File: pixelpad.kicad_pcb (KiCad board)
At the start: 2 copper layers, 19 x 57 mm, 4 parts, among them SW1 SW_Push, SW2 SW_Push, SW3 SW_Push, U1 MOUDLE-SEEEDUINO-XIAO

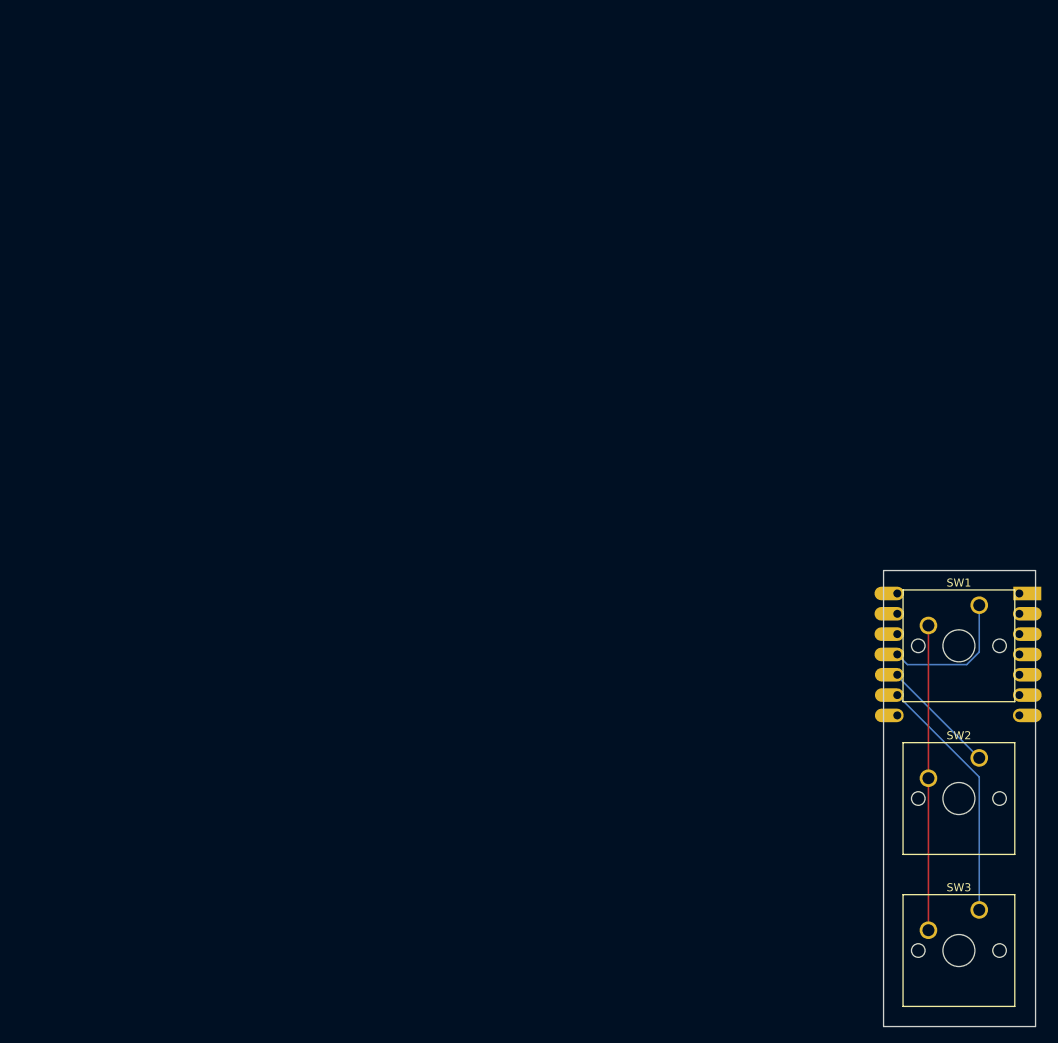
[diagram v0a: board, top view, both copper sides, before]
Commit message: Added stuff to the pcb editor
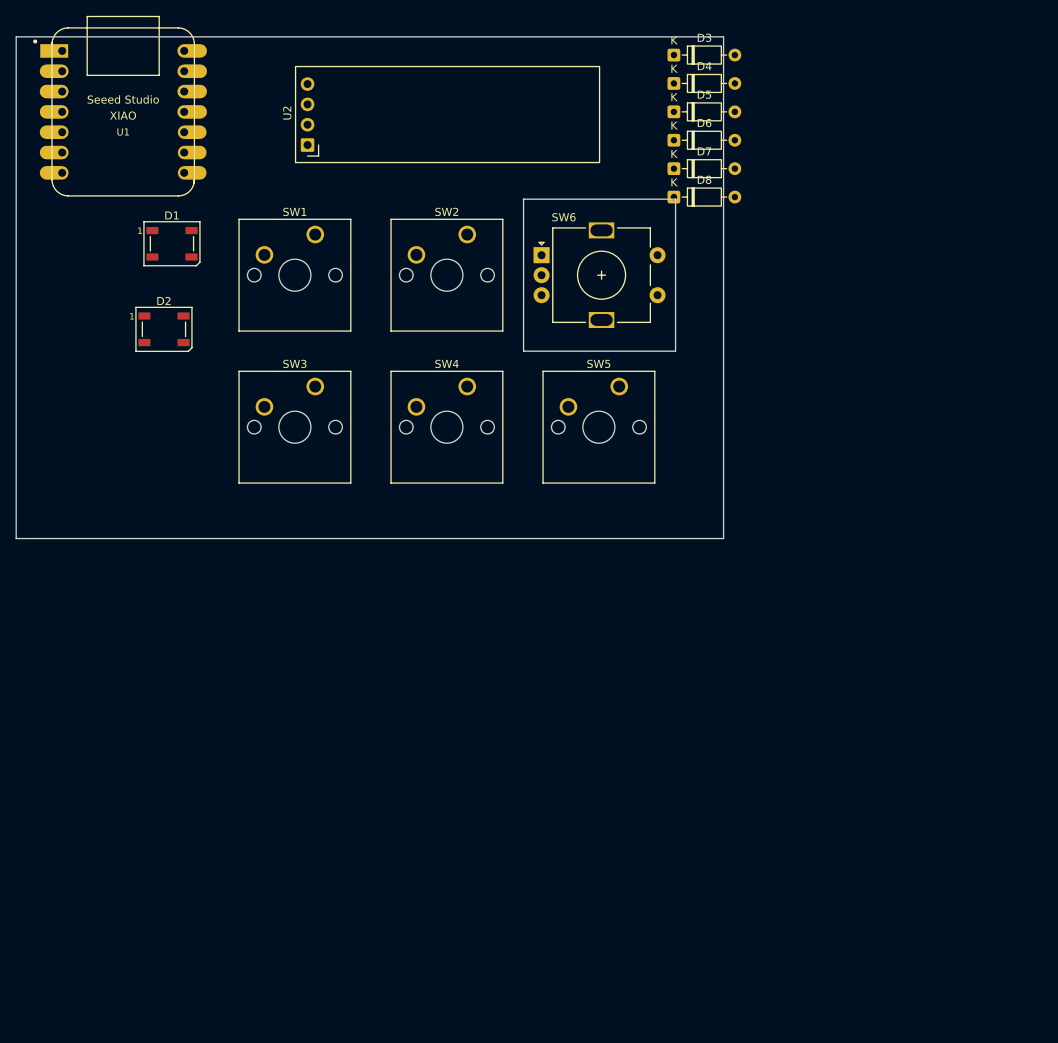
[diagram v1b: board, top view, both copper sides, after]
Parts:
- added D1: WS2812B, LED_SMD:LED_WS2812B_PLCC4_5.0x5.0mm_P3.2mm, F.Cu at (56.5, 45.1)
- added D2: WS2812B, LED_SMD:LED_WS2812B_PLCC4_5.0x5.0mm_P3.2mm, F.Cu at (55.5, 55.9)
- added D3: 1N914, Diode_THT:D_DO-35_SOD27_P7.62mm_Horizontal, F.Cu at (119.3, 21.6)
- added D4: 1N914, Diode_THT:D_DO-35_SOD27_P7.62mm_Horizontal, F.Cu at (119.3, 25.1)
- added D5: 1N914, Diode_THT:D_DO-35_SOD27_P7.62mm_Horizontal, F.Cu at (119.3, 28.7)
- added D6: 1N914, Diode_THT:D_DO-35_SOD27_P7.62mm_Horizontal, F.Cu at (119.3, 32.2)
- added D7: 1N914, Diode_THT:D_DO-35_SOD27_P7.62mm_Horizontal, F.Cu at (119.3, 35.8)
- added D8: 1N914, Diode_THT:D_DO-35_SOD27_P7.62mm_Horizontal, F.Cu at (119.3, 39.3)
- added SW4: SW_Push_45deg, Button_Switch_Keyboard:SW_Cherry_MX_1.00u_PCB, F.Cu at (93.5, 63.0)
- added SW5: SW_Push_45deg, Button_Switch_Keyboard:SW_Cherry_MX_1.00u_PCB, F.Cu at (112.5, 63.0)
- added SW6: RotaryEncoder_Switch, Rotary_Encoder:RotaryEncoder_Alps_EC11E-Switch_Vertical_H20mm, F.Cu at (102.8, 46.6)
- added U2: ER_OLEDM0.91_1x-I2C, Display:ER_OLEDM0.91_1x-I2C, F.Cu at (73.5, 32.8)
- SW1, SW2, SW3: value SW_Push -> SW_Push_45deg
- U1: moved to F.Cu
- moved U1 124.5 mm to (50.5, 28.7), turned to 0 degrees
- moved SW3 105.7 mm to (74.5, 63.0)
- moved SW1 95.1 mm to (74.5, 44.0)
- moved SW2 91.5 mm to (93.5, 44.0)
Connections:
- SW1 pad 1: Net-(U1-PA6_A10_D10_MOSI) -> COL0
- SW1 pad 2: GND -> Net-(D4-A)
- SW2 pad 1: Net-(U1-PA5_A9_D9_MISO) -> COL1
- SW2 pad 2: GND -> Net-(D5-A)
- SW3 pad 1: Net-(U1-PA7_A8_D8_SCK) -> COL2
- SW3 pad 2: GND -> Net-(D8-A)
- U1 pad 1: unconnected-(U1-PA02_A0_D0-Pad1) -> COL1
- U1 pad 10: Net-(U1-PA5_A9_D9_MISO) -> COL2
- U1 pad 11: Net-(U1-PA6_A10_D10_MOSI) -> unconnected-(U1-PA6_A10_D10_MOSI-Pad11)
- U1 pad 14: unconnected-(U1-5V-Pad14) -> VCC
- U1 pad 2: unconnected-(U1-PA4_A1_D1-Pad2) -> COL0
- U1 pad 3: unconnected-(U1-PA10_A2_D2-Pad3) -> ROW1
- U1 pad 4: unconnected-(U1-PA11_A3_D3-Pad4) -> ROW0
- U1 pad 5: unconnected-(U1-PA8_A4_D4_SDA-Pad5) -> SDA
- U1 pad 6: unconnected-(U1-PA9_A5_D5_SCL-Pad6) -> SCL
- U1 pad 8: unconnected-(U1-PB09_A7_D7_RX-Pad8) -> EC11B
- U1 pad 9: Net-(U1-PA7_A8_D8_SCK) -> EC11A
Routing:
- net GND: track 38.1 -> 0.00 mm
- net Net-(U1-PA7_A8_D8_SCK): track 31.1 -> 0.00 mm
- net Net-(U1-PA6_A10_D10_MOSI): track 17.6 -> 0.00 mm
- net Net-(U1-PA5_A9_D9_MISO): track 14.6 -> 0.00 mm
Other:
- board size 19 x 57 mm -> 88.4 x 62.7 mm

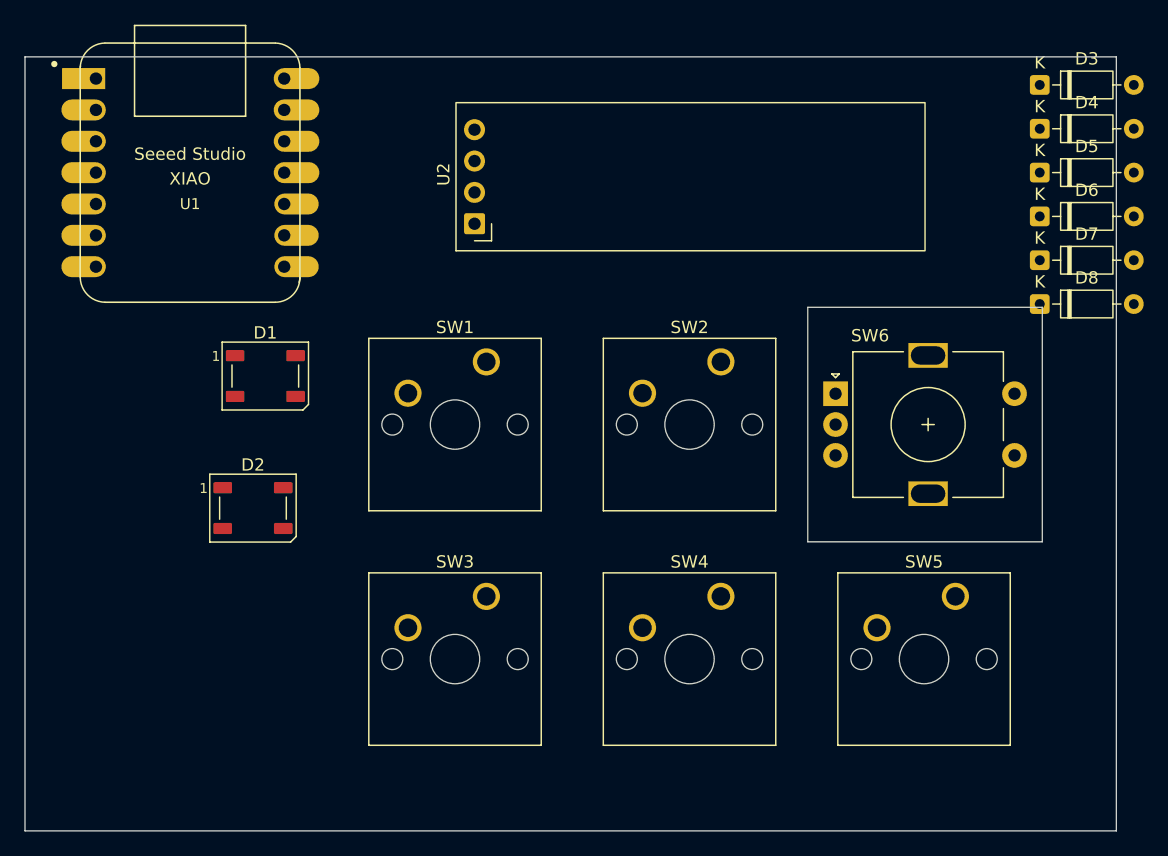
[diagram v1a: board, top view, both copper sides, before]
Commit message: Fully wired up!
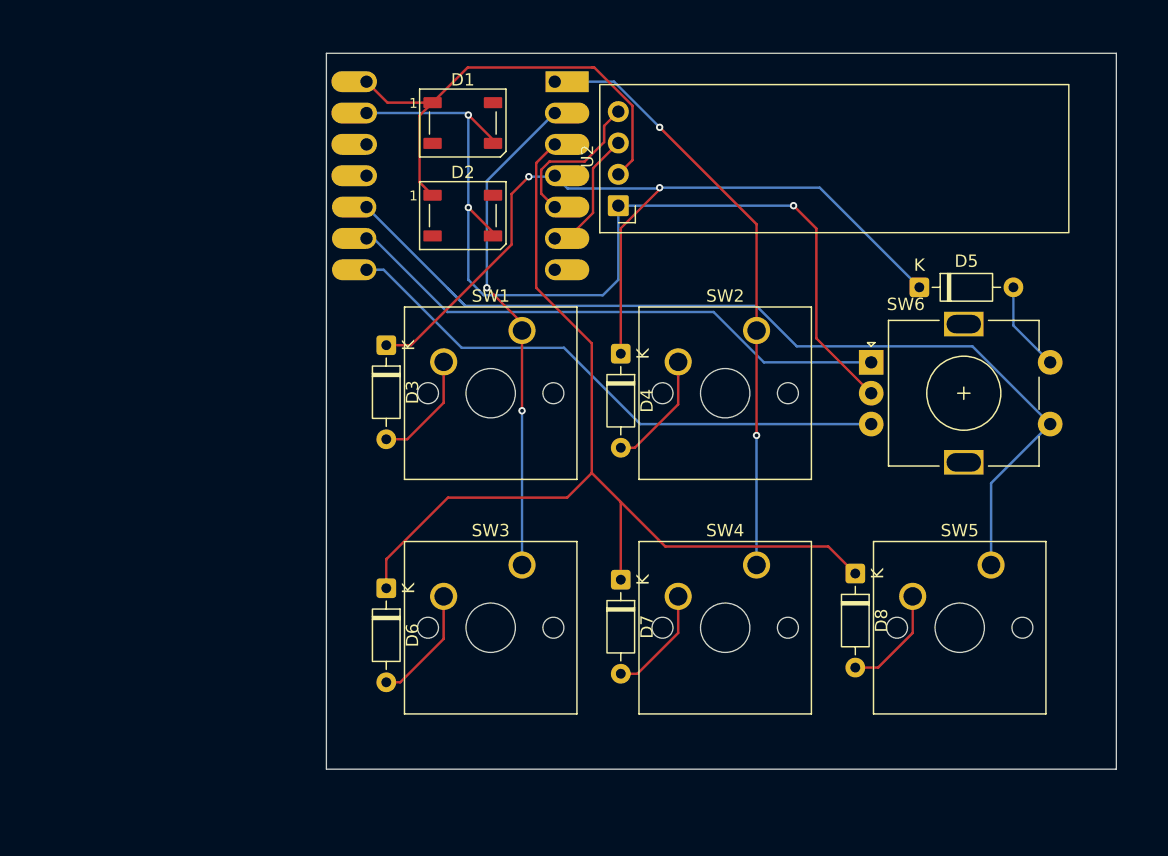
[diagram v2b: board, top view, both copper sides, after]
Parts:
- U1: moved to B.Cu
- moved D6 59.2 mm to (66.3, 62.3), turned to -90 degrees
- moved D3 55.8 mm to (66.3, 42.6), turned to -90 degrees
- moved D7 44.9 mm to (85.3, 61.6), turned to -90 degrees
- moved D4 37.0 mm to (85.3, 43.3), turned to -90 degrees
- moved D2 29.2 mm to (72.5, 32.1)
- moved D8 26.5 mm to (104.3, 61.1), turned to -90 degrees
- moved D1 26.0 mm to (72.5, 24.6)
- moved U1 21.9 mm to (72.4, 28.9), turned to 180 degrees
- moved D5 19.1 mm to (109.5, 38.0)
- moved U2 11.7 mm to (85.2, 31.3)
- moved SW1 3.85 mm to (77.3, 41.5)
- moved SW2 3.85 mm to (96.3, 41.5)
- moved SW3 3.85 mm to (77.3, 60.5)
- moved SW4 3.85 mm to (96.3, 60.5)
- moved SW5 3.85 mm to (115.3, 60.5)
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- renumbered D4 to D3, D5 to D4, D3 to D5, D7 to D6, D6 to D7
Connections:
- D6 pad 2: Net-(D7-A) -> Net-(D6-A)
- D7 pad 2: Net-(D6-A) -> Net-(D7-A)
- SW3 pad 1: COL2 -> COL0
- SW3 pad 2: Net-(D8-A) -> Net-(D6-A)
- SW4 pad 1: COL0 -> COL1
- SW5 pad 1: COL1 -> COL2
- SW5 pad 2: Net-(D6-A) -> Net-(D8-A)
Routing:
- net ROW1: track 0.00 -> 82.1 mm
- net GND: track 0.00 -> 79.3 mm, vias 0 -> 3
- net COL2: track 0.00 -> 78.1 mm
- net ROW0: track 0.00 -> 69.8 mm, vias 0 -> 2
- net COL1: track 0.00 -> 48.7 mm, vias 0 -> 2
- net EC11B: track 0.00 -> 46.1 mm
- net EC11A: track 0.00 -> 45.0 mm
- net COL0: track 0.00 -> 40.1 mm, vias 0 -> 2
- net VCC: track 0.00 -> 39.1 mm
- net SDA: track 0.00 -> 12.4 mm
- net SCL: track 0.00 -> 10.5 mm
- net Net-(D4-A): track 0.00 -> 9.55 mm
- net Net-(D6-A): track 0.00 -> 9.55 mm
- net Net-(D3-A): track 0.00 -> 9.19 mm
- net Net-(D7-A): track 0.00 -> 8.99 mm
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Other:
- board size 88.4 x 62.7 mm -> 64 x 58 mm
